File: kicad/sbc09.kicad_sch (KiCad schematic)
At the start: 77 parts, among them J1 Conn_01x04_Male, J2 Conn_01x06_Male, J3 Conn_01x06_Male, J4 Conn_01x06_Male, J5 Conn_02x05_Odd_Even, J6 Conn_02x25_Odd_Even, J7 Conn_02x05_Odd_Even, Q1 2N7000, SW1 SW_Push, U1 74HCT245, U10 SST39SF040-DIP, U11 XR68C681CJ, U12 MAX232, U2 74HCT245, U3 74HCT245, U4 MC6809E, U5 74HCT32, U6 EPM7128SLC84, U7 71256SA15TPG, U8 AS6C4008-55PCN, U9 SST39SF040-DIP, X1 8MHz, X2 3.6864MHz

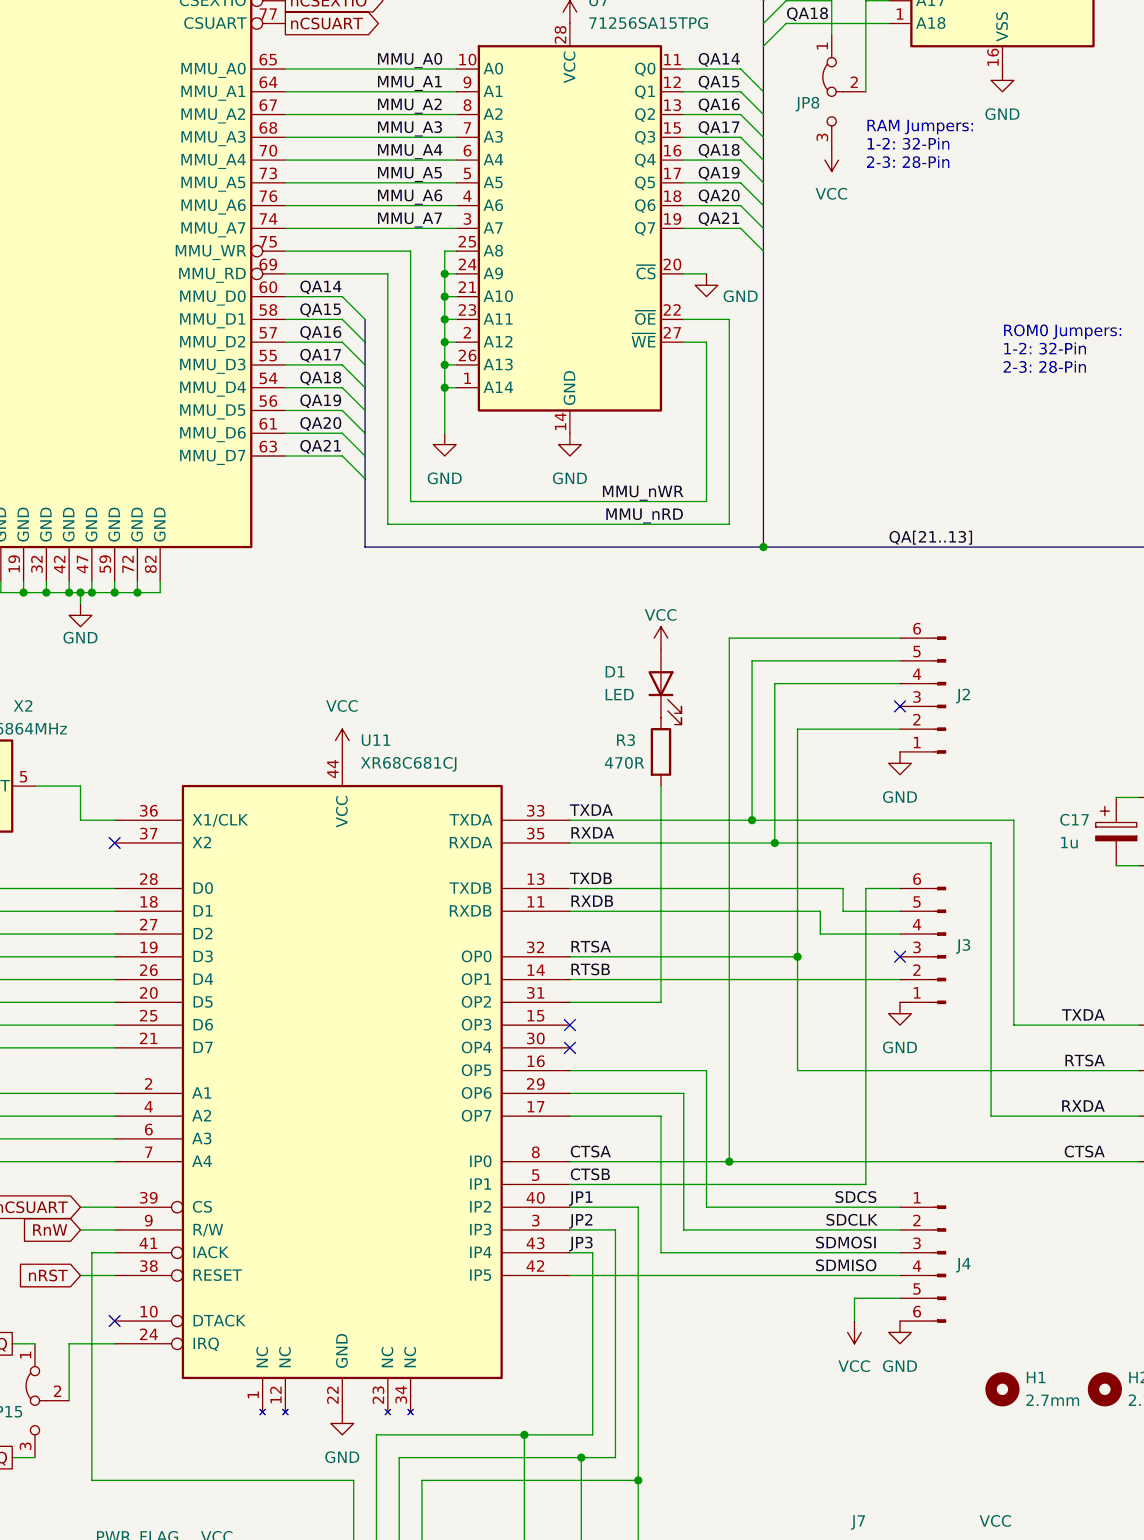
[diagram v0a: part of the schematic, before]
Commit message: KiCAD: Connect SD Card to CPLD
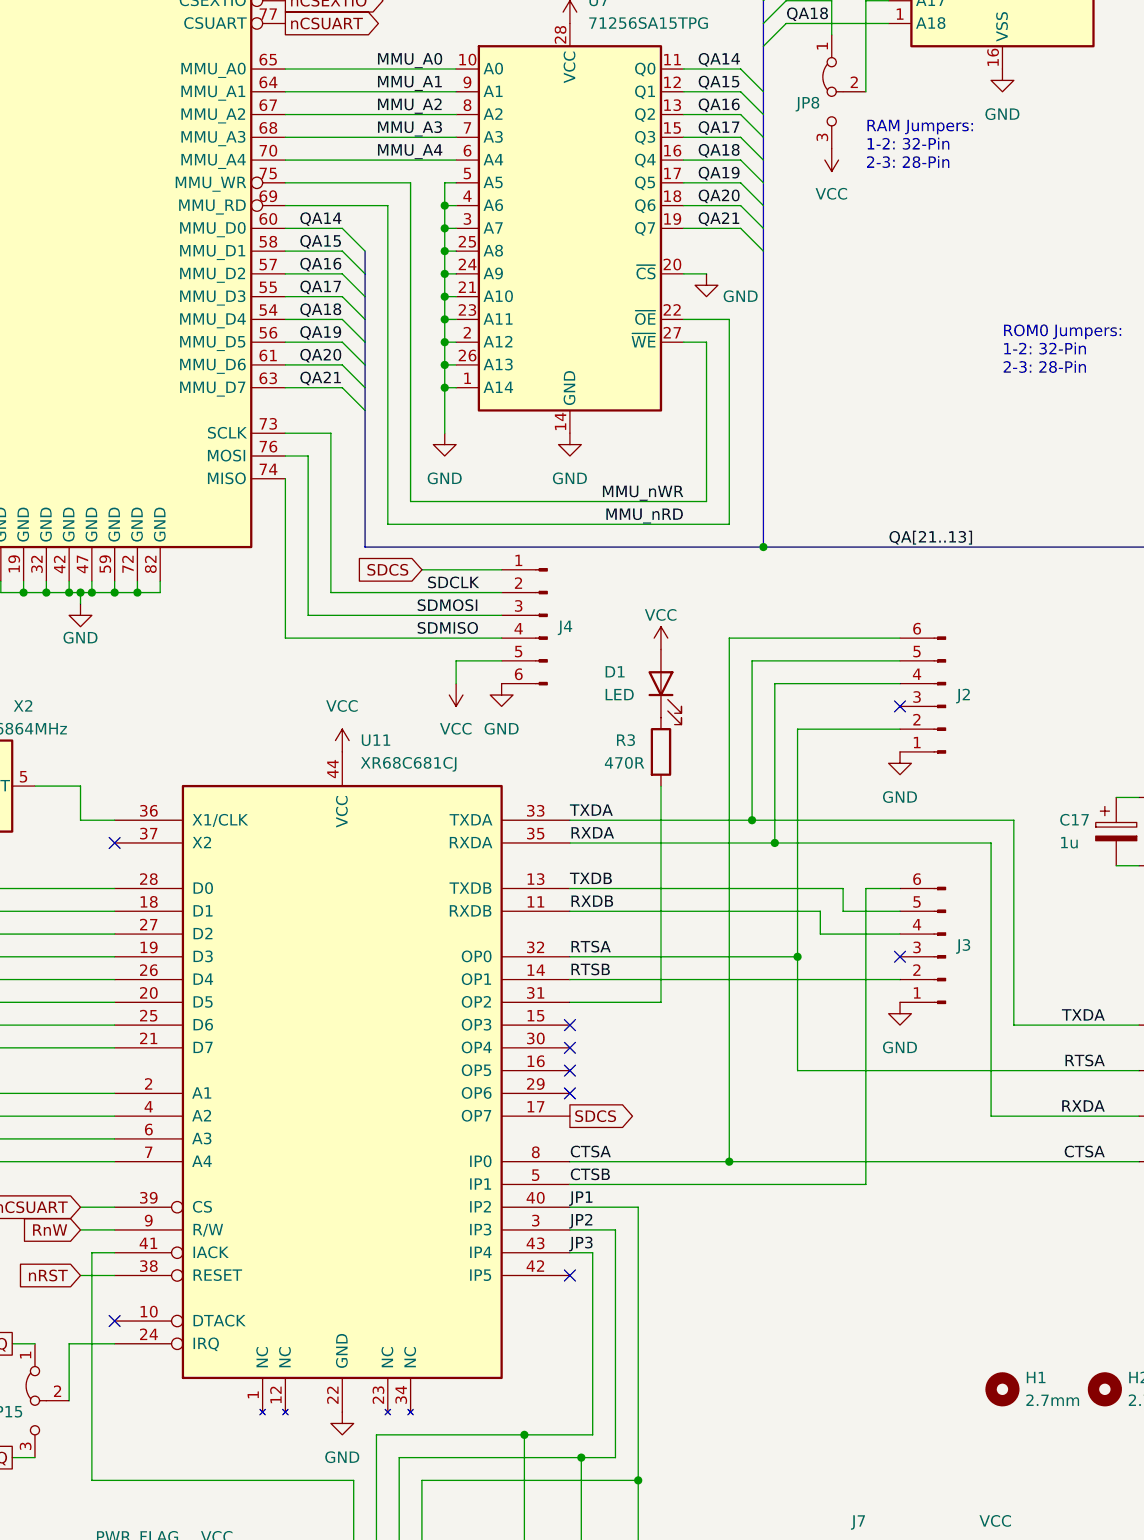
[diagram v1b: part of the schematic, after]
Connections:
- net GND: now also U7.3 (A7), U7.4 (A6), U7.5 (A5)
- net SDCLK: now also U6.73 (SCLK); no longer U11.29 (OP6)
- net SDCS: now also U11.17 (OP7); no longer U11.16 (OP5)
- net SDMISO: now also U6.74 (MISO); no longer U11.42 (IP5)
- net SDMOSI: now also U6.76 (MOSI); no longer U11.17 (OP7)
- removed net MMU_A5: U6.73 (MMU_A5), U7.5 (A5)
- removed net MMU_A6: U6.76 (MMU_A6), U7.4 (A6)
- removed net MMU_A7: U6.74 (MMU_A7), U7.3 (A7)
- no-connect marks 21 -> 24
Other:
- moved on the sheet: J4
